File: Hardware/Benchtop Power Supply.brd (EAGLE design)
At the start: 114.3 x 48.3 mm, 20 parts, among them J1 ATX24RH

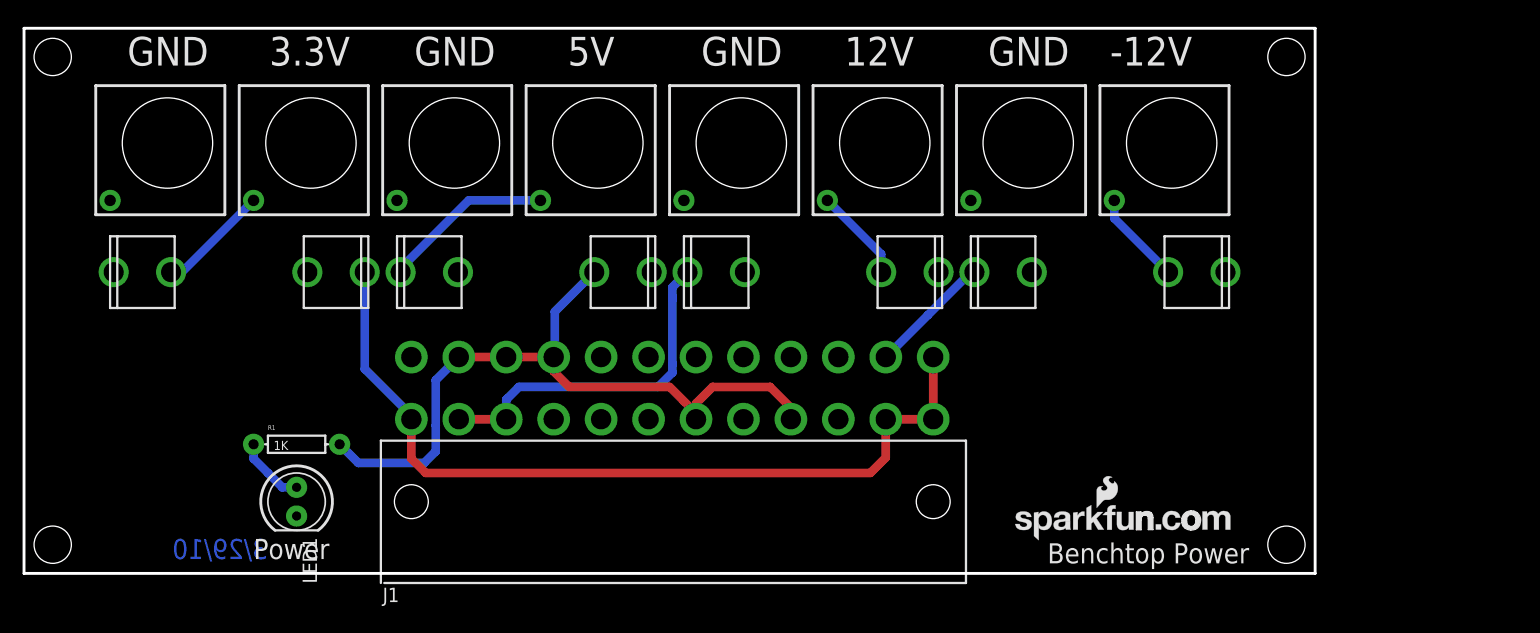
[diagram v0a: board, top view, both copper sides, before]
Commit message: Midway hardware changes
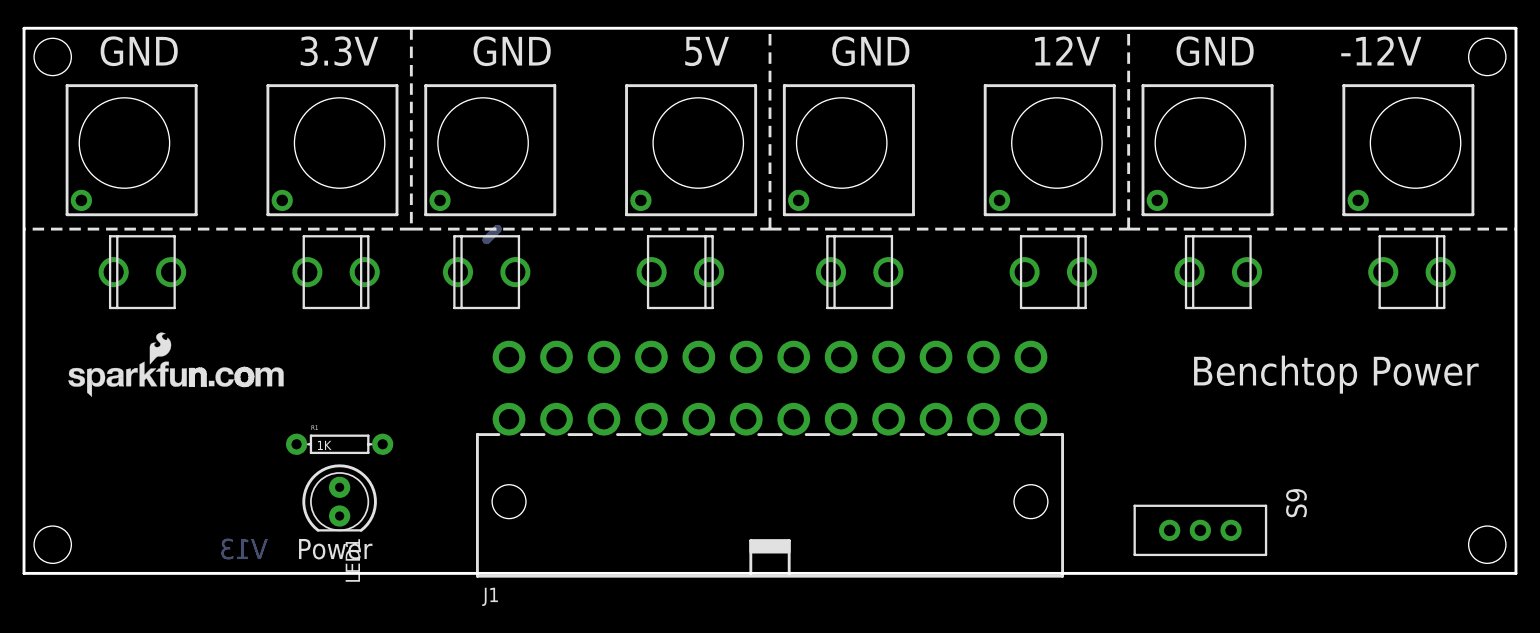
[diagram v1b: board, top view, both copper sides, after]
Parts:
- added FRAME1: FRAME-LETTER, SparkFun-Aesthetics:CREATIVE_COMMONS
- added S9: (no value), SparkFun-Electromechanical:SWITCH-SPDT_KIT
- added U$1: REVISION, SparkFun-Aesthetics:REVISION
- J1: device SparkFun:ATX24_RIGHT_ANGLE -> SparkFun-Connectors:ATX24_RIGHT_ANGLE
- moved JP1 84.8 mm to (3.94, 15.6)
- moved S8 21.6 mm to (123.2, 38.1)
- moved F4 19.0 mm to (114.3, 26.7)
- moved JP2 17.8 mm to (129.5, 2.54)
- moved JP3 17.8 mm to (129.5, 45.7)
- moved S6 15.2 mm to (91.4, 38.1)
- moved S7 15.2 mm to (104.1, 38.1)
- moved F3 12.7 mm to (82.5, 26.7)
- moved J1 8.89 mm to (66.0, 8.89)
- moved S4 8.89 mm to (59.7, 38.1)
- moved S5 8.89 mm to (72.4, 38.1)
- moved F1 5.08 mm to (49.5, 26.7)
- moved LED1 3.81 mm to (27.9, 6.35)
- moved R1 3.81 mm to (27.9, 11.4)
- moved S1 3.81 mm to (8.89, 38.1)
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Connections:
- new net N$2: J1.16, S9.2
- net GND: now also S9.3; no longer J1.16
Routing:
- net 3.3V: track 74.7 -> 0.00 mm
- net 5V: track 64.8 -> 0.00 mm
- net 12V: track 31.4 -> 0.00 mm
- net 5V_P: track 15.2 -> 1.35 mm
- net -12V: track 11.0 -> 0.00 mm
- net 3.3V_P: track 9.93 -> 0.95 mm
- net -12V_P: track 8.32 -> 0.00 mm
- net 12V_P: track 8.32 -> 0.00 mm
- net N$1: track 6.13 -> 0.00 mm
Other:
- board size 114.3 x 48.3 mm -> 132.1 x 48.3 mm
- board text added: "Ryan Owens"
- board text added: "Toni Klopfenstein"
- board text added: "V13"
- board text removed: "3/29/10"
